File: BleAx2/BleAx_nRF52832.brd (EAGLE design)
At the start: 30 x 20.1 mm, 42 parts, among them CN1 6p-2.54, J1 2.0MM-90D, U1 NRF52832, U2 MCP73832T-2ACI/OT-SOT23-5, U4 MIC5225-3.3, X1 FA-128, X2 32.768kHz

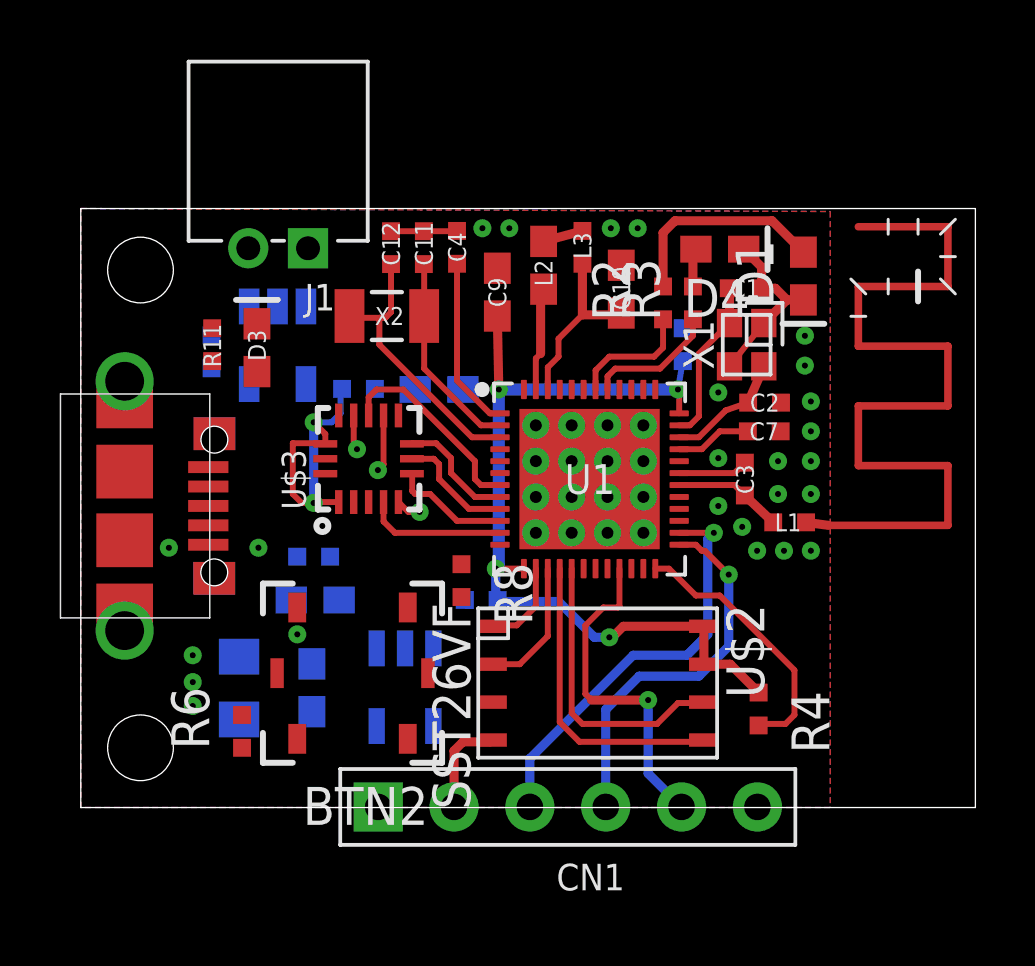
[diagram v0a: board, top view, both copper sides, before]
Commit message: pred_auto
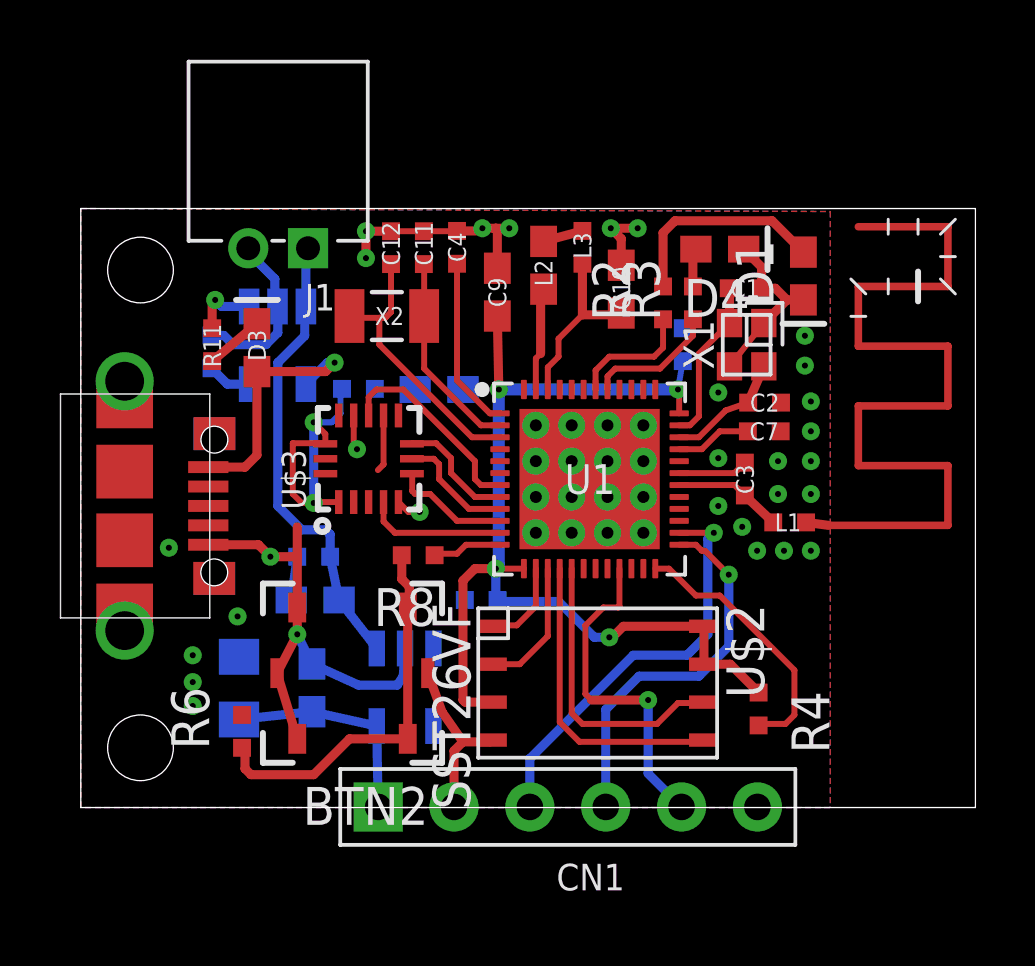
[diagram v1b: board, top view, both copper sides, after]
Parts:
- moved R8 1.68 mm to (11.3, 8.45), turned to 180 degrees
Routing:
- net GND: track 17.9 -> 50.8 mm, vias 28 -> 30
- net VDD_BATT: track 0.00 -> 15.5 mm
- net VDD_P3V3: track 39.4 -> 53.1 mm
- net N$6: track 0.00 -> 13.0 mm
- net VCC_P5V0_USB: track 0.00 -> 8.58 mm, vias 0 -> 1
- net N$10: track 0.00 -> 2.51 mm, vias 0 -> 1
- net BTTN_01: track 0.00 -> 2.33 mm
- net N$9: track 0.00 -> 1.95 mm
- net N$1: track 0.00 -> 1.48 mm
